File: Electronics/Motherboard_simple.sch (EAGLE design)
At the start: 27 parts

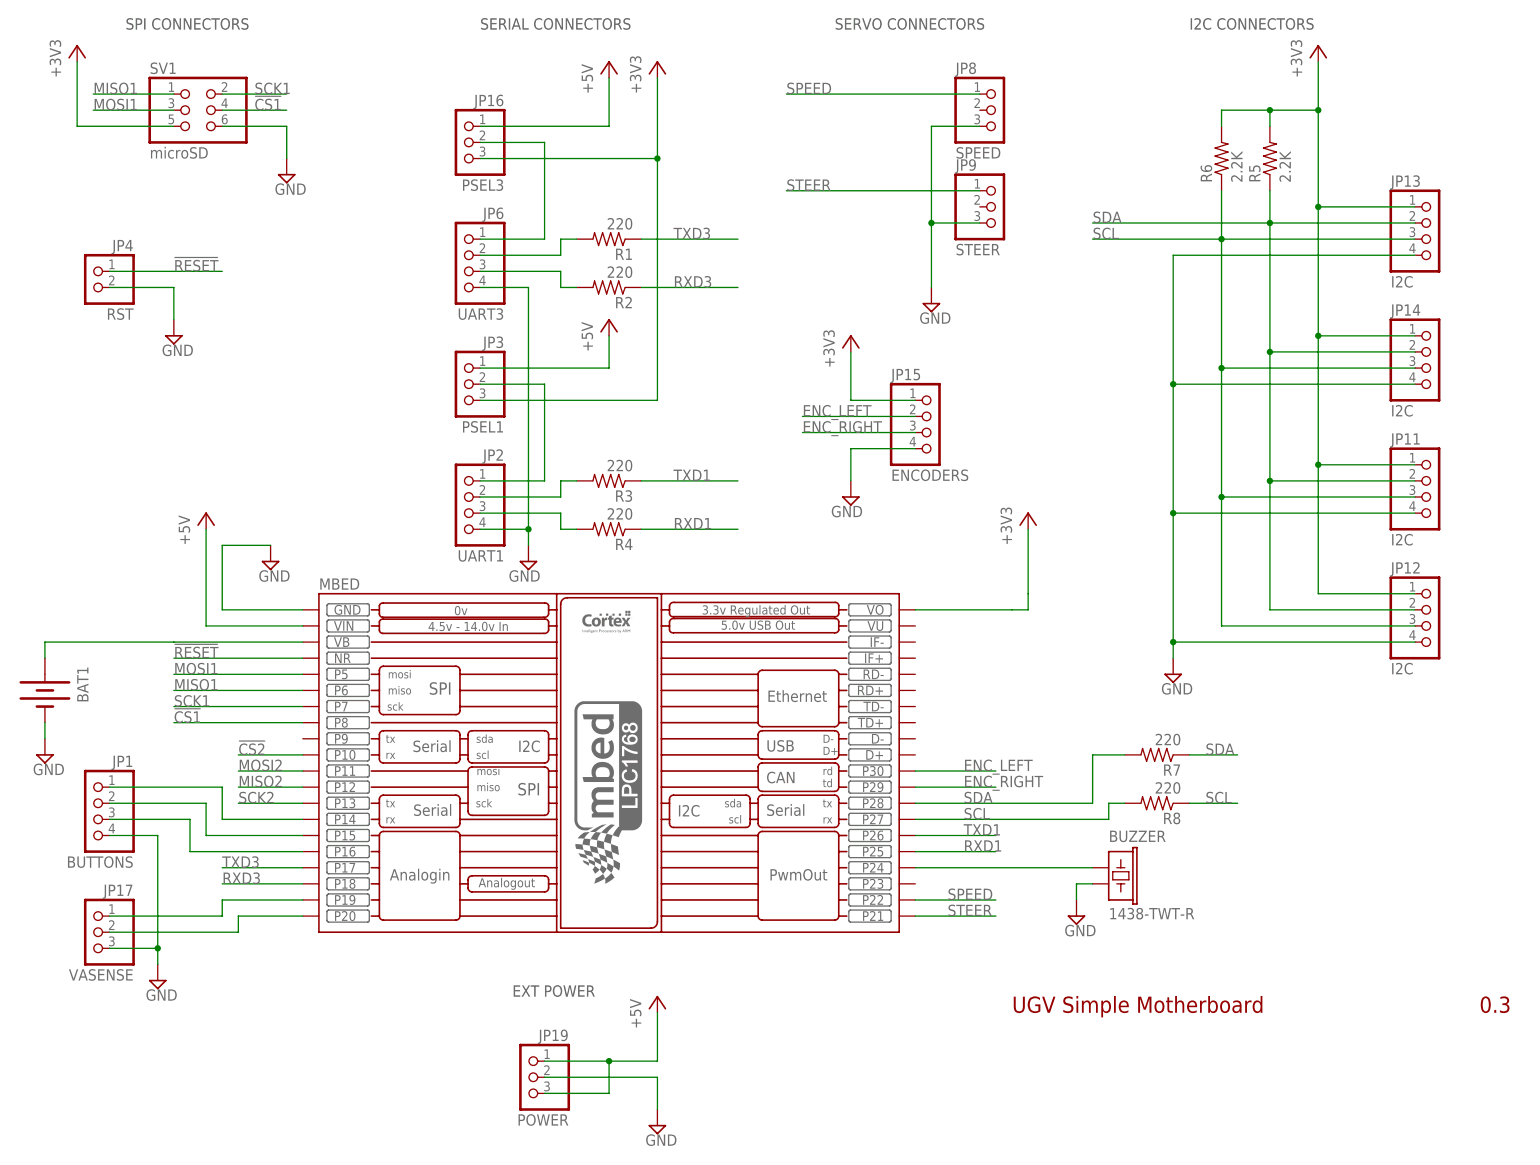
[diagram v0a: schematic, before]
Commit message: Minor updates and tweaks
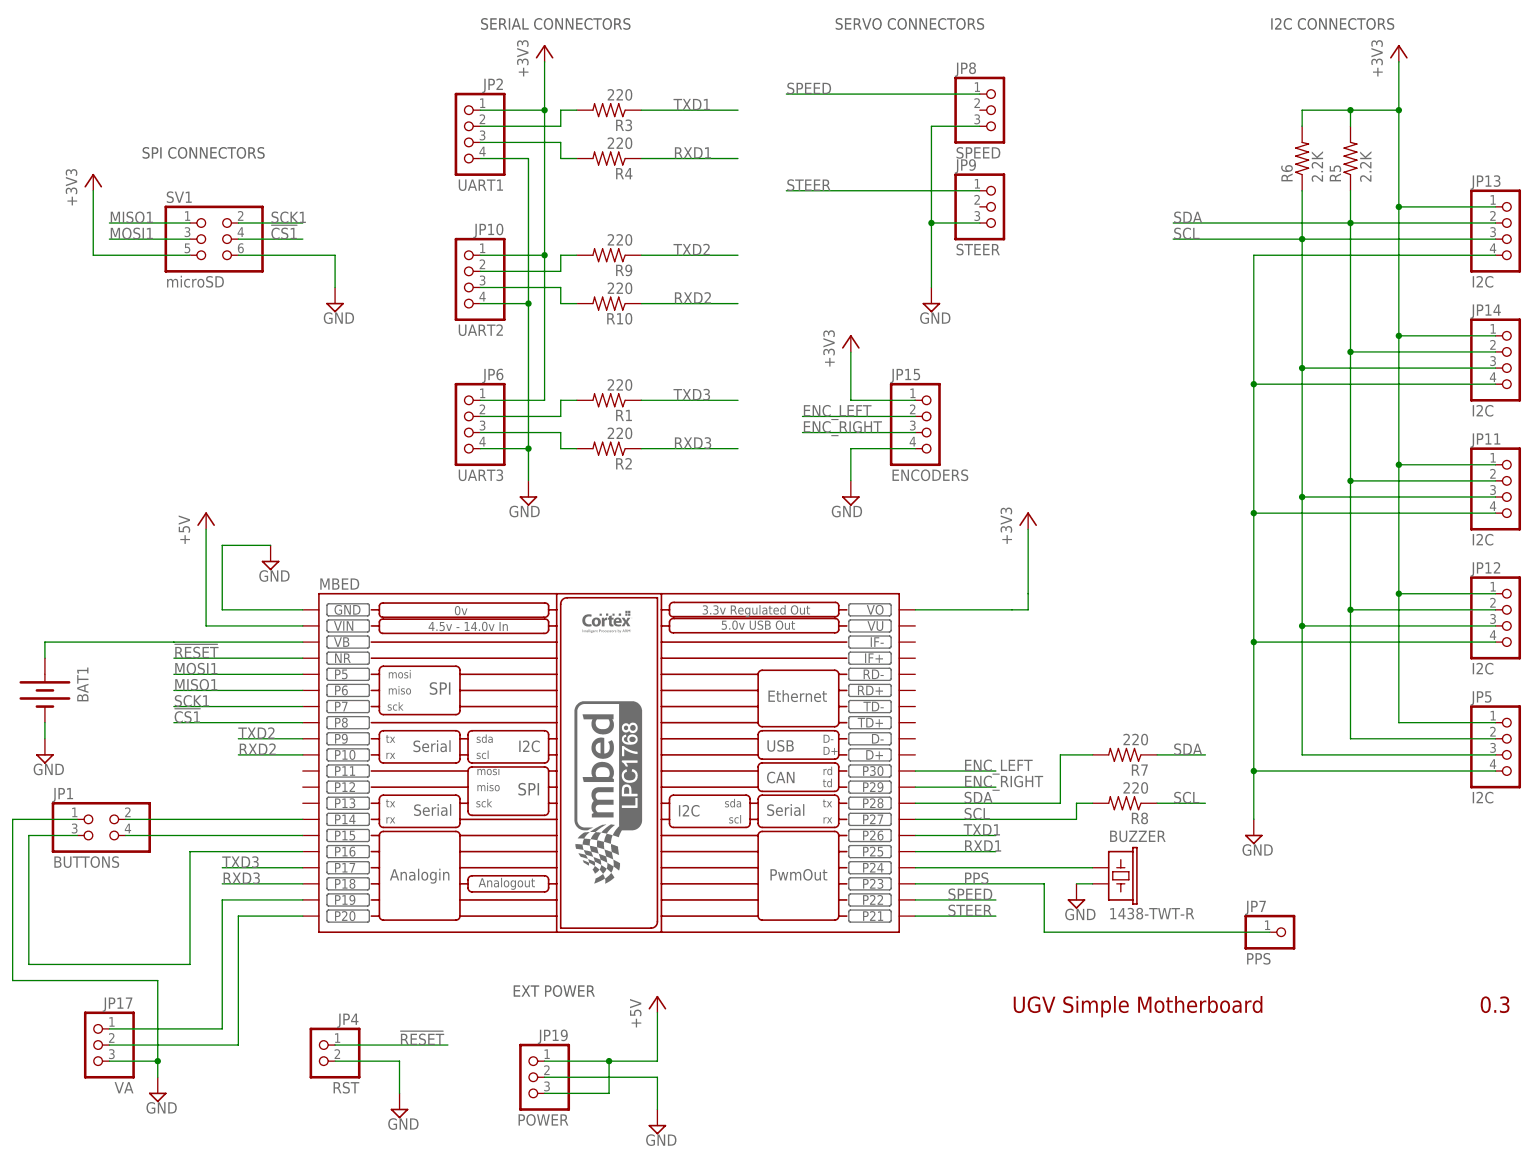
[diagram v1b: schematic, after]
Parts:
- removed JP16: PSEL3, pinhead-2:PINHD-1X03_2.54-S
- removed JP3: PSEL1, pinhead-2:PINHD-1X03_2.54-S
- added JP10: UART2, pinhead-2:PINHD-1X04_2.54-S
- added JP5: I2C, pinhead-2:PINHD-1X04_2.54-S
- added JP7: PPS, pinhead-2:PINHD-1X01_2.54-S
- added R10, R9: 220, rcl:R-US_R0805
- BAT1: device SparkFun:BATTERY12PTH -> SparkFun:BATTERY12MM
- JP1: device pinhead-2:PINHD-1X04_2.54-S -> pinhead-2:PINHD-2X02_2.54; OC_NEWARK unknown -> (none)
- JP17: value VASENSE -> VA
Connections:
- removed net !CS2: MBED.P10
- removed net MISO2: MBED.P12
- removed net MOSI2: MBED.P11
- removed net N$11: JP2.1, JP3.2
- removed net N$3: JP16.2, JP6.1
- removed net SCK2: MBED.P13
- new net N$16: JP10.2, R9.2
- new net N$17: JP10.3, R10.2
- new net PPS: JP7.1, MBED.P23
- new net RXD2: MBED.P10, R10.1
- new net TXD2: MBED.P9, R9.1
- net +3V3: now also JP10.1, JP2.1, JP5.1, JP6.1; no longer JP16.3, JP3.3
- net +5V: no longer JP16.1, JP3.1
- net GND: now also JP1.1, JP10.4, JP5.4; no longer JP1.4
- net N$5: now also JP1.2; no longer JP1.1
- net N$7: now also JP1.4; no longer JP1.2
- net SCL: now also JP5.3
- net SDA: now also JP5.2
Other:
- moved on the sheet: JP1, JP11, JP12, JP13, JP14, JP17, JP2, JP4, JP6, R1, R2, R3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
